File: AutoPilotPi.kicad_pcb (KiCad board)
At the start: 4 copper layers, 29 x 44.7 mm, 105 parts, among them J1 Conn_01x04_MountingPin, J2 Conn_01x04_MountingPin, J3 Conn_01x04_MountingPin, J4 USB_C_Receptacle, SW1 SW_Push, U1 MKDV4GCL-AB, U2 V3S-ALLWINNER, U3 EA3036, U4 GW1N_LV4QN32C6/I5, U5 HMC5883L-TR, U6 SPL06-001, U7 v3s_flight_controller, U8 TLV71312PDBV, Y1 Crystal, Y2 Crystal_GND24_Small

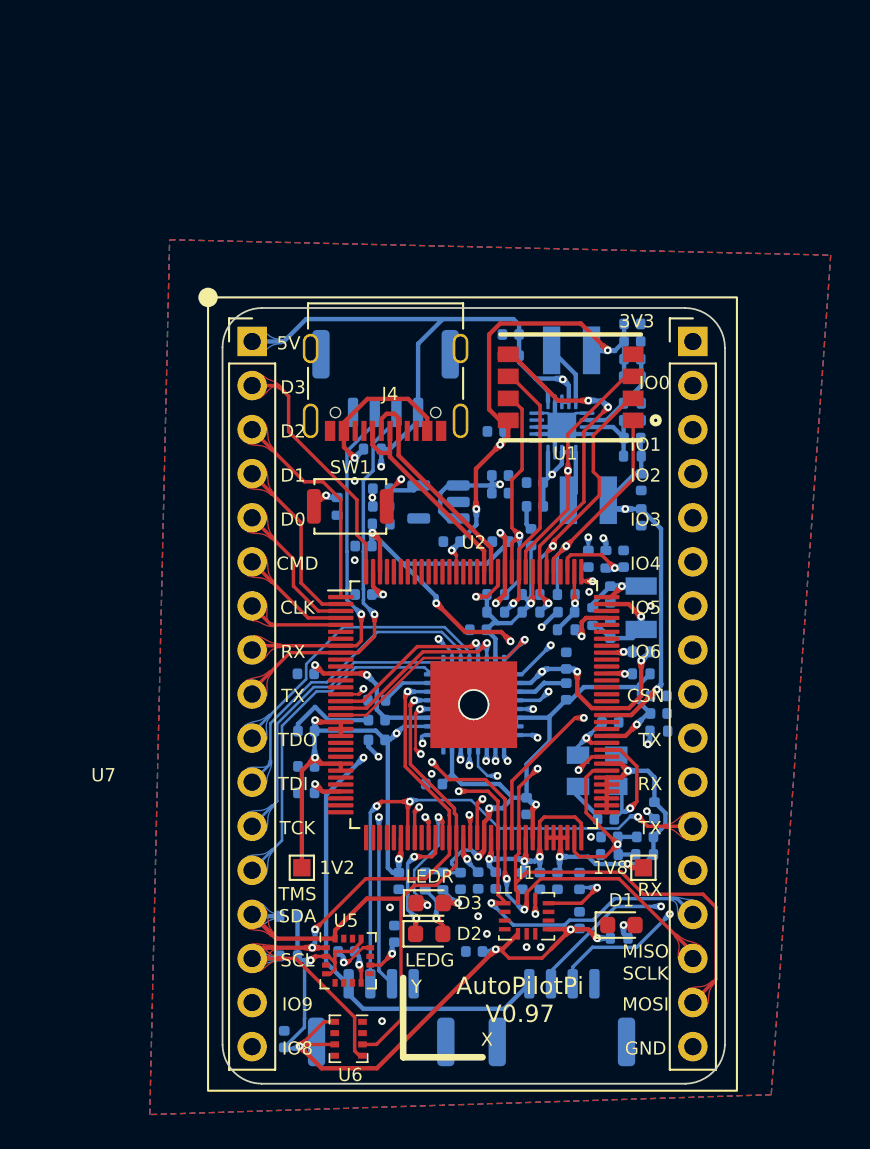
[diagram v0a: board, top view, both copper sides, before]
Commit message: update mini
Signed-off-by: huangzzk <huangcmzzk@gmail.com>
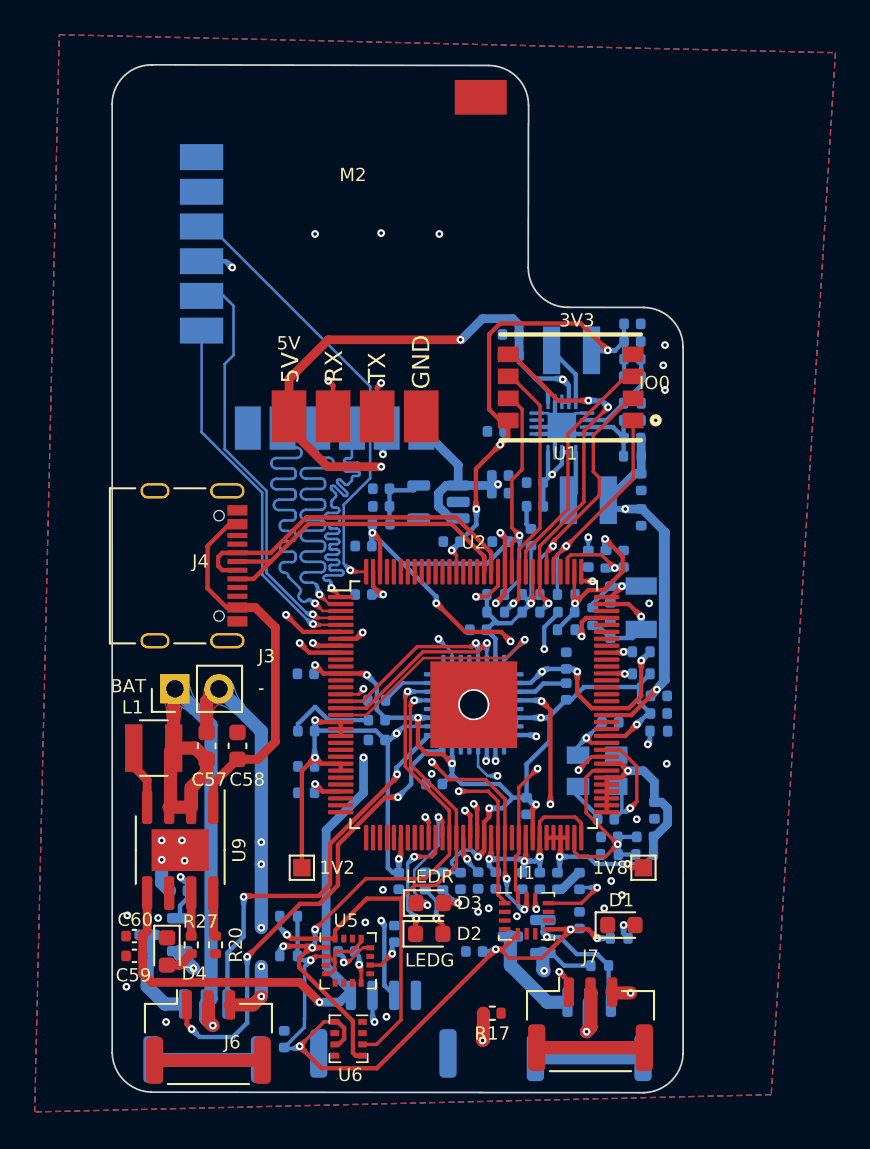
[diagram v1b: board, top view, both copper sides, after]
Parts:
- removed SW1: SW_Push, Button_Switch_SMD:SW_Push_SPST_NO_Alps_SKRK
- removed U7: v3s_flight_controller, ic_footprint:Flight_Core
- added C57: 10u, Capacitor_SMD:C_0603_1608Metric, F.Cu at (77.1, 71.5)
- added C58: 10u, Capacitor_SMD:C_0603_1608Metric, F.Cu at (78.8, 71.5)
- added C59: 1u, Capacitor_SMD:C_0402_1005Metric, F.Cu at (72.9, 83.6)
- added C60: 0.1u, Capacitor_SMD:C_0402_1005Metric, F.Cu at (72.9, 82.4)
- added D4: LED, LED_SMD:LED_0603_1608Metric, F.Cu at (74.8, 83.3)
- added J5: Conn_01x03, Connector_Molex:Molex_CLIK-Mate_502386-0370_1x03-1MP_P1.25mm_Horizontal, B.Cu at (99.1, 88.1)
- added J6: Conn_01x03, Connector_Molex:Molex_CLIK-Mate_502386-0370_1x03-1MP_P1.25mm_Horizontal, F.Cu at (77.2, 88.2)
- added J7: Conn_01x03, Connector_Molex:Molex_CLIK-Mate_502386-0370_1x03-1MP_P1.25mm_Horizontal, F.Cu at (99.2, 87.5)
- added L1: L, Inductor_SMD:L_Abracon_ASPI-3012S, F.Cu at (74.0, 71.6)
- added M1: xr819, ic_footprint:xr819_module, B.Cu at (84.5, 44.9)
- added M2: mini_elrs, ic_footprint:mini_elrs, F.Cu at (84.9, 38.2)
- added Q1: Q_NMOS_GSD, Package_TO_SOT_SMD:SOT-23, B.Cu at (74.6, 82.3)
- added Q2: Q_NMOS_GSD, Package_TO_SOT_SMD:SOT-23, B.Cu at (95.5, 82.4)
- added R17: 0R, Resistor_SMD:R_0402_1005Metric, F.Cu at (93.5, 86.9)
- added R28: 10K, Resistor_SMD:R_0402_1005Metric, B.Cu at (75.4, 79.8)
- added R29: 10K, Resistor_SMD:R_0402_1005Metric, B.Cu at (99.7, 84.1)
- added U9: ETA9640, Package_SO:SOIC-8-1EP_3.9x4.9mm_P1.27mm_EP2.41x3.3mm, F.Cu at (75.5, 77.5)
- C11, C12, C17, C18: value 18pf -> 18p
- C15: value 1uF -> 1u
- C31, C34: value 4.7uF -> 4.7u
- C51: value 0.22uF -> 0.22u
- J2: value Conn_01x04_MountingPin -> Conn_01x03; footprint Connector_Molex:Molex_CLIK-Mate_502382-0470_1x04-1MP_P1.25mm_Vertical -> Connector_Molex:Molex_CLIK-Mate_502386-0370_1x03-1MP_P1.25mm_Horizontal
- J3: value Conn_01x04_MountingPin -> Conn_01x02; footprint Connector_Molex:Molex_CLIK-Mate_502382-0470_1x04-1MP_P1.25mm_Vertical -> Connector_PinHeader_2.54mm:PinHeader_1x02_P2.54mm_Vertical; moved to F.Cu
- R20: value 0R -> 1.2k; moved to F.Cu
- R21: value 10K -> 0R
- R23: value 4.7k -> 4.7K
- R27: value 499R -> 10K; moved to F.Cu
- U8: value TLV71312PDBV -> ME6212C12M5G
- moved J2 39.3 mm to (77.0, 88.2)
- moved R20 30.0 mm to (77.6, 82.9), turned to -90 degrees
- moved R27 26.6 mm to (76.2, 82.9), turned to 90 degrees
- moved J3 22.4 mm to (75.2, 68.2), turned to 90 degrees
- moved J4 15.1 mm to (76.3, 61.1), turned to -90 degrees
- moved J1 10.3 mm to (87.2, 87.8)
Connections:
- J2 pad 1: +5V -> /FPGAIO5
- J2 pad 2: /U1_TX -> +BATT
- J2 pad 3: /U1_RX -> Net-(Q1-Pad3)
- J2 pad MP: GND -> (no net)
- J3 pad 1: +5V -> +BATT
- J3 pad 2: /U2_TX -> GNDPWR
- R20 pad 1: +5V -> Net-(R20-Pad1)
- R20 pad 2: VBUS -> GND
- R27 pad 2: GND -> Net-(R27-Pad2)
- U2 pad 6: unconnected-(U2-Pad6) -> /WIRQ
- U2 pad 7: unconnected-(U2-Pad7) -> /WREST
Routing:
- net GNDPWR: track 0.00 -> 76.4 mm, vias 0 -> 13
- net +BATT: track 0.00 -> 65.9 mm, vias 0 -> 2
- net +3V3: track 159.9 -> 203.9 mm, vias 21 -> 25
- net /U2_TX: track 32.1 -> 0.00 mm, vias 3 -> 0
- net /U2_RX: track 31.6 -> 0.00 mm, vias 2 -> 0
- net /FPGAIO7: track 0.00 -> 27.3 mm, vias 0 -> 3
- net /WIRQ: track 0.00 -> 26.8 mm, vias 0 -> 2
- net /FPGAIO8: track 25.3 -> 0.00 mm, vias 1 -> 0
- net (no net): track 0.00 -> 24.8 mm
- net +1V8: track 63.9 -> 87.0 mm
- net /FPGAIO6: track 22.4 -> 0.00 mm, vias 2 -> 0
- net /FPGAIO9: track 22.4 -> 0.00 mm, vias 1 -> 0
- net /FPGAIO0: track 21.1 -> 0.00 mm, vias 1 -> 0
- net /FPGAIO4: track 20.0 -> 0.00 mm, vias 1 -> 0
- net /FPGAIO2: track 19.5 -> 0.00 mm, vias 1 -> 0
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- removed copper zone on In2.Cu, net GND
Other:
- board size 29 x 44.7 mm -> 32.9 x 59.2 mm
- board text added: "-"
- board text added: "BAT"
- board text removed: "AutoPilotPi V0.97"
- board text removed: "CLK"
- board text removed: "CMD"
- board text removed: "CSN"
- board text removed: "D0"
- board text removed: "D1"
- board text removed: "D2"
- board text removed: "D3"
- board text removed: "GND"
- board text removed: "IO1"
- board text removed: "IO2"
- board text removed: "IO3"
- board text removed: "IO4"
- board text removed: "IO5"
- board text removed: "IO6"
- board text removed: "IO8"
- board text removed: "IO9"
- board text removed: "MISO"
- board text removed: "MOSI"
- board text removed: "SCL"
- board text removed: "SCLK"
- board text removed: "SDA"
- board text removed: "TCK"
- board text removed: "TDI"
- board text removed: "TDO"
- board text removed: "TMS"
- board text removed: "U2"
- board text removed: "X"
- board text removed: "Y"
